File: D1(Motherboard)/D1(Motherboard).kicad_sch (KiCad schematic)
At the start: 50 parts, among them J1 WR-FPC_0.5mm_ZIF_V, J2 USB_C_Receptacle_USB2.0, J3 B2B-PH-K-S, Q1 NX2301P.215, SW1 CHS-02A, U1 CP2102N-A01-GQFN28, U2 ICM-20602, U3 WR-FPC_0.5mm_ZIF_H, U4 MIC5353-3.3YMT, U5 FAN5331SX, U6 MCP73831-2-OT

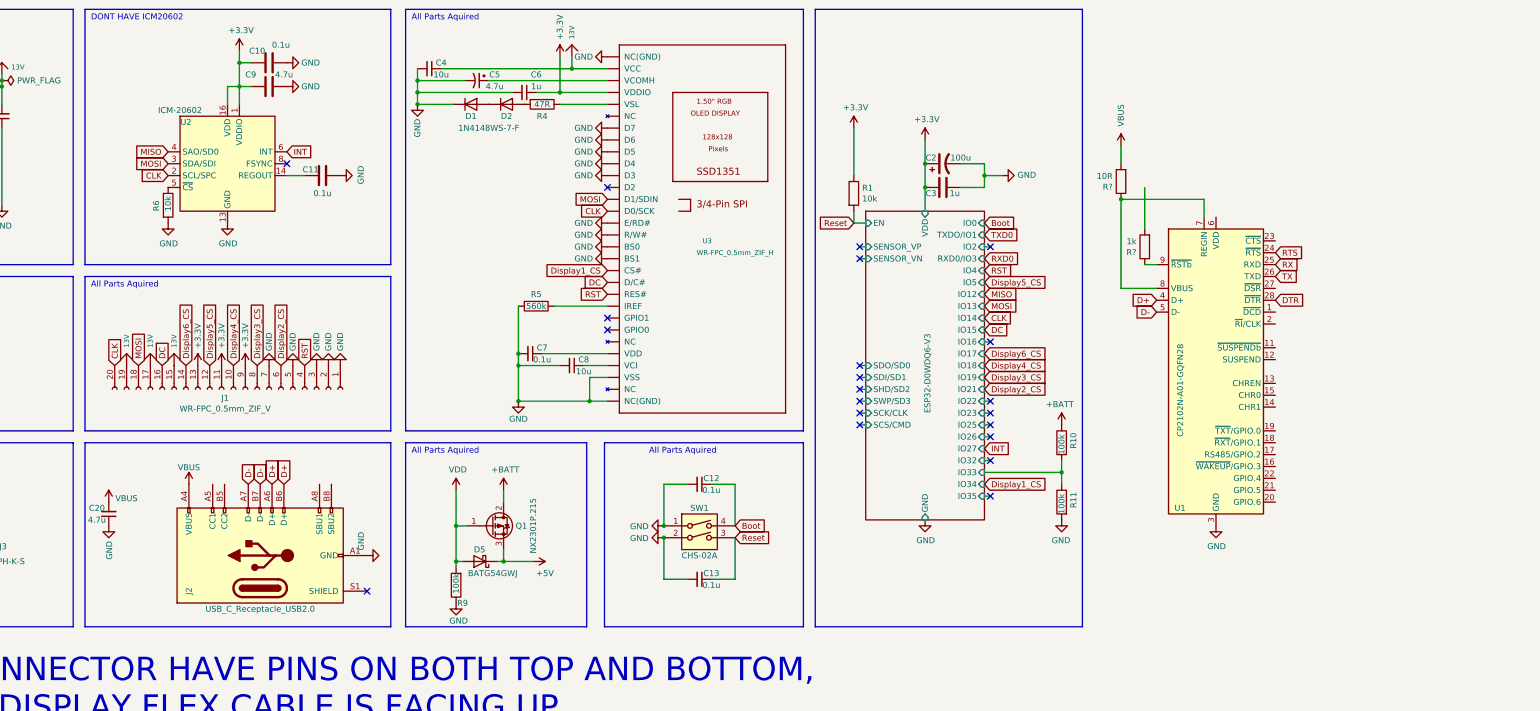
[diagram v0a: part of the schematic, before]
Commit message: Test Commit for CADLAB
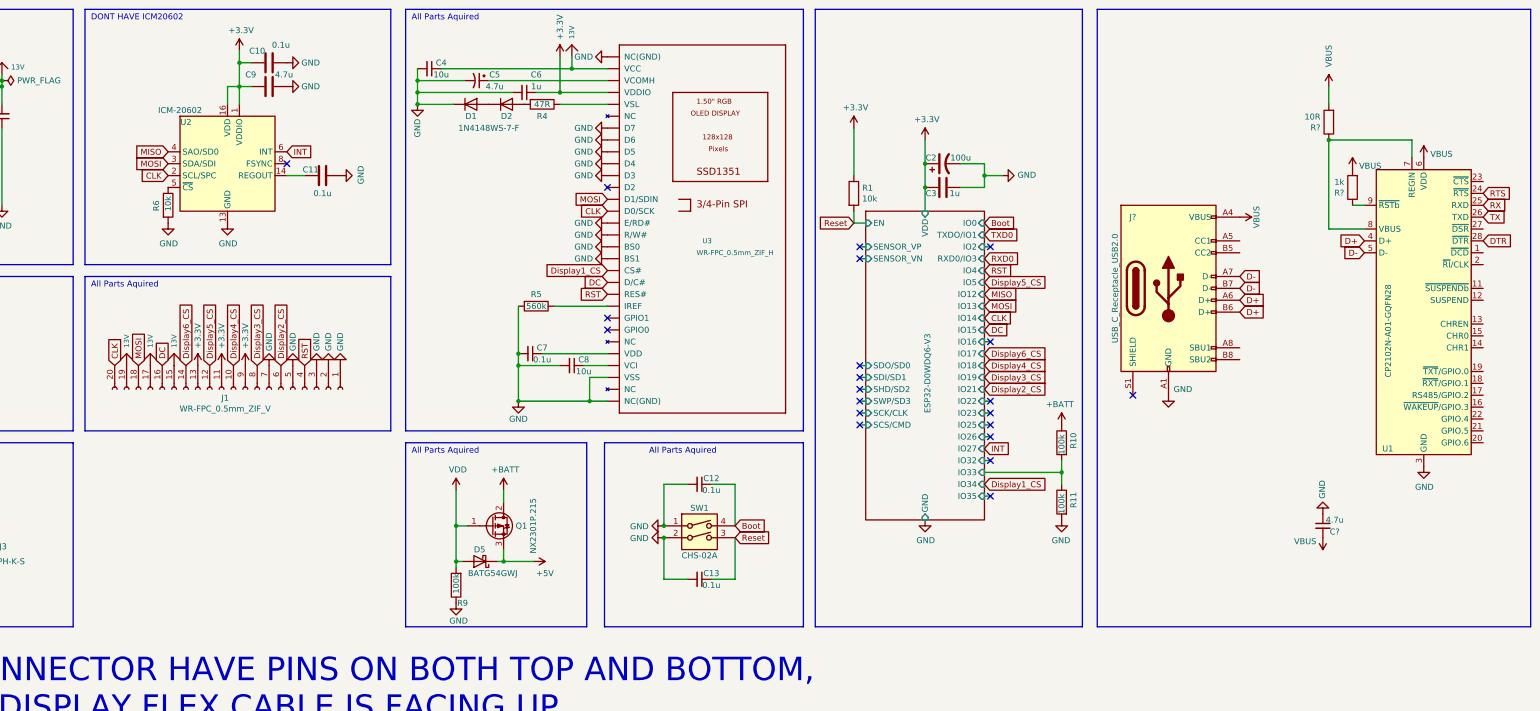
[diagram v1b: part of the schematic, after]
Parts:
- removed C20: 4.7u, Capacitor_SMD:C_0603_1608Metric, symbol Device:C_Small
- removed J2: USB_C_Receptacle_USB2.0, Connector_USB:USB_C_Receptacle_JAE_DX07S024WJ3R400, symbol Connector:USB_C_Receptacle_USB2.0
- added C?: 4.7u, Capacitor_SMD:C_0603_1608Metric, symbol Device:C_Small
- added J?: USB_C_Receptacle_USB2.0, Connector_USB:USB_C_Receptacle_JAE_DX07S024WJ3R400, symbol Connector:USB_C_Receptacle_USB2.0
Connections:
- net D+: now also J?.A6 (D+), J?.B6 (D+)
- net D-: now also J?.A7 (D-), J?.B7 (D-)
- net GND: now also C?.1, J?.A1 (GND), J?.A12 (GND), J?.B1 (GND), J?.B12 (GND)
- net VBUS: now also R?.2, U1.6 (VDD), C?.2, J?.A4 (VBUS), J?.A9 (VBUS), J?.B4 (VBUS), J?.B9 (VBUS)
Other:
- moved on the sheet: R?, U1
